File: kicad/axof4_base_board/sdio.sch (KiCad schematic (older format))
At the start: 0 parts

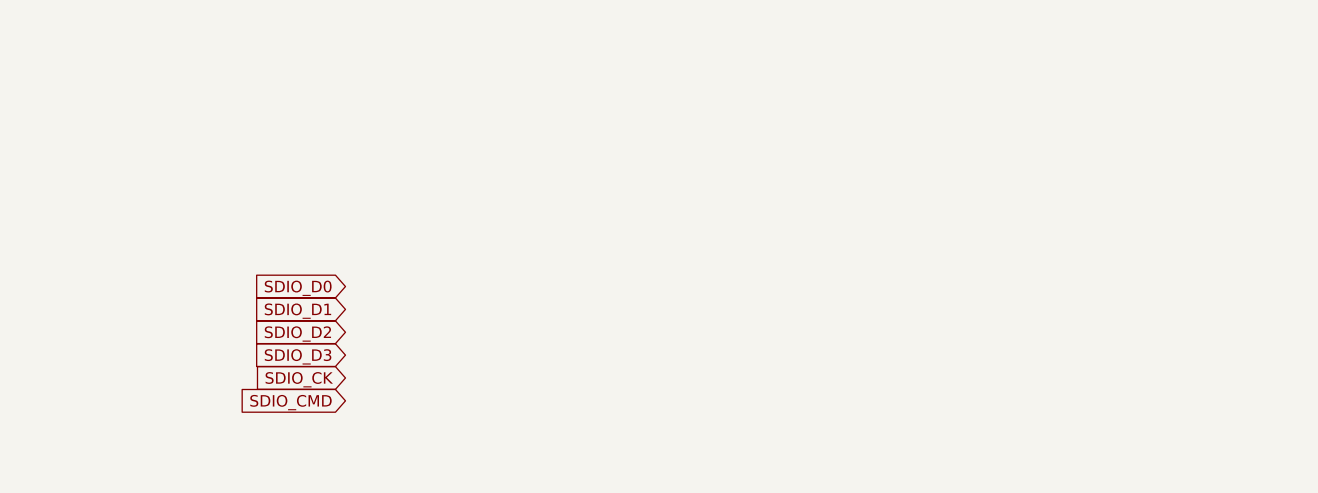
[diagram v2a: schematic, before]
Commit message: cleanup, dedicated PCB WIP
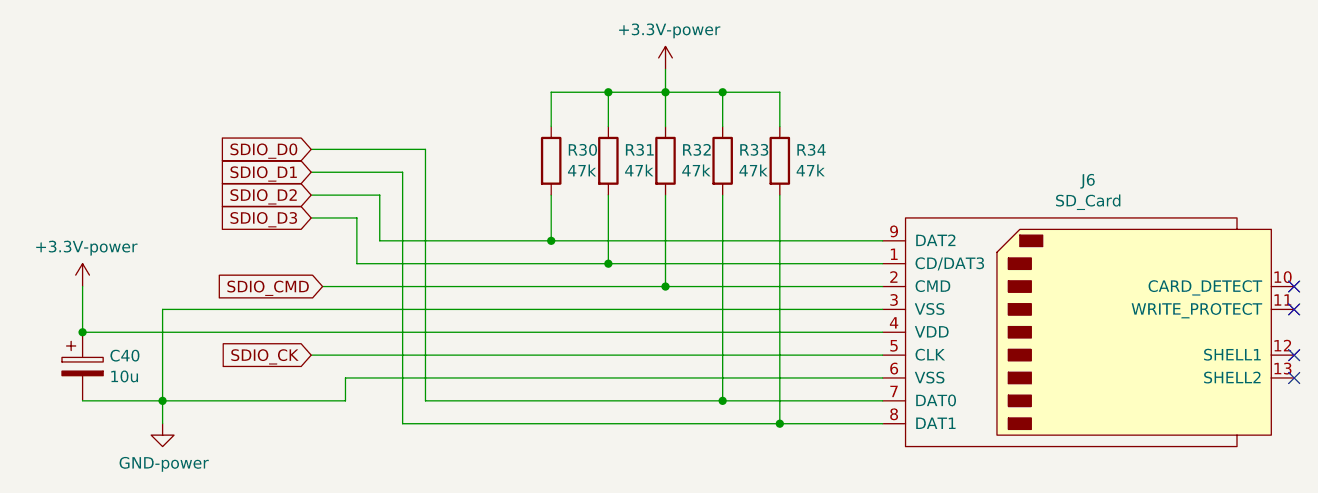
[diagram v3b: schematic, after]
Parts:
- added C40: 10u, Capacitor_SMD:CP_Elec_4x5.4, symbol Device:CP
- added J6: SD_Card, Connector_Card:SD_TE_2041021, symbol Connector:SD_Card
- added R30, R31, R32, R33, R34: 47k, Resistor_SMD:R_1206_3216Metric_Pad1.42x1.75mm_HandSolder, symbol Device:R
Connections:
- net SDIO_CK: now also J6.5 (CLK)
- net SDIO_CMD: now also J6.2 (CMD), R32.2
- net SDIO_D0: now also J6.7 (DAT0), R33.2
- net SDIO_D1: now also J6.8 (DAT1), R34.2
- net SDIO_D2: now also J6.9 (DAT2), R30.2
- net SDIO_D3: now also J6.1 (CD/DAT3), R31.2
- new net +3V3: C40.1, J6.4 (VDD), R30.1, R31.1, R32.1, R33.1, R34.1
- new net GND: C40.2, J6.3 (VSS), J6.6 (VSS)
- no-connect marks 0 -> 4
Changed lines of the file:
@@
 $Descr A4 11693 8268
 encoding utf-8
-Sheet 3 6
+Sheet 3 7
 Title ""
 Date ""
@@
 Comment4 ""
 $EndDescr
-Text GLabel 2500 2700 0    50   Input ~ 0
+Text GLabel 2350 2100 0    50   Input ~ 0
 SDIO_D0
-Text GLabel 2500 2800 0    50   Input ~ 0
+Text GLabel 2350 2200 0    50   Input ~ 0
 SDIO_D1
-Text GLabel 2500 2900 0    50   Input ~ 0
+Text GLabel 2350 2300 0    50   Input ~ 0
 SDIO_D2
-Text GLabel 2500 3000 0    50   Input ~ 0
+Text GLabel 2350 2400 0    50   Input ~ 0
 SDIO_D3
-Text GLabel 2500 3100 0    50   Input ~ 0
+Text GLabel 2400 2700 0    50   Input ~ 0
+SDIO_CMD
+$Comp
+L Connector:SD_Card J6
+U 1 1 5F740056
+P 5750 2900
+F 0 "J6" H 5750 3565 50  0000 C CNN
+F 1 "SD_Card" H 5750 3474 50  0000 C CNN
+F 2 "Connector_Card:SD_TE_2041021" H 5750 2900 50  0001 C CNN
+F 3 "http://portal.fciconnect.com/Comergent//fci/drawing/10067847.pdf" H 5750 2900 50  0001 C CNN
+	1    5750 2900
+	1    0    0    -1
+$EndComp
+Text GLabel 2350 3000 0    50   Input ~ 0
 SDIO_CK
-Text GLabel 2500 3200 0    50   Input ~ 0
-SDIO_CMD
+Wire Wire Line
+	2350 3000 4850 3000
+Wire Wire Line
+	2400 2700 3900 2700
+Wire Wire Line
+	2350 2100 2850 2100
+Wire Wire Line
+	2850 2100 2850 3200
+Wire Wire Line
+	2850 3200 4150 3200
+Wire Wire Line
+	2350 2200 2750 2200
+Wire Wire Line
+	2750 2200 2750 3300
+Wire Wire Line
+	2750 3300 4400 3300
+Wire Wire Line
+	2350 2300 2650 2300
+Wire Wire Line
+	2650 2300 2650 2500
+Wire Wire Line
+	2350 2400 2550 2400
+Wire Wire Line
+	2550 2400 2550 2600
+Wire Wire Line
+	2550 2600 3650 2600
+$Comp
+L axof4_base_board-rescue:+3.3V-power #PWR0103
+U 1 1 5F743FB7
+P 1350 2700
+F 0 "#PWR0103" H 1350 2550 50  0001 C CNN
+F 1 "+3.3V-power" H 1365 2873 50  0000 C CNN
+F 2 "" H 1350 2700 50  0001 C CNN
+F 3 "" H 1350 2700 50  0001 C CNN
+	1    1350 2700
+	1    0    0    -1
+$EndComp
+$Comp
+L axof4_base_board-rescue:GND-power #PWR0104
+U 1 1 5F744B0D
+P 1700 3300
+F 0 "#PWR0104" H 1700 3050 50  0001 C CNN
+F 1 "GND-power" H 1705 3127 50  0000 C CNN
+F 2 "" H 1700 3300 50  0001 C CNN
+F 3 "" H 1700 3300 50  0001 C CNN
+	1    1700 3300
+	1    0    0    -1
+$EndComp
+Wire Wire Line
+	1700 3300 1700 3200
+Wire Wire Line
+	1700 2800 4850 2800
+Wire Wire Line
+	1350 2700 1350 2900
+Wire Wire Line
+	1350 2900 4850 2900
+NoConn ~ 6650 2700
+NoConn ~ 6650 2800
+NoConn ~ 6650 3000
+NoConn ~ 6650 3100
+$Comp
+L Device:CP C40
+U 1 1 5F750B90
+P 1350 3050
+F 0 "C40" H 1468 3096 50  0000 L CNN
+F 1 "10u" H 1468 3005 50  0000 L CNN
+F 2 "Capacitor_SMD:CP_Elec_4x5.4" H 1388 2900 50  0001 C CNN
+F 3 "~" H 1350 3050 50  0001 C CNN
+	1    1350 3050
+	1    0    0    -1
+$EndComp
+Connection ~ 1350 2900
+Wire Wire Line
+	1350 3200 1700 3200
+Connection ~ 1700 3200
+Wire Wire Line
+	1700 2800 1700 3200
+Wire Wire Line
+	1700 3200 2500 3200
+Wire Wire Line
+	2500 3200 2500 3100
+Wire Wire Line
+	2500 3100 4850 3100
+$Comp
+L Device:R R30
+U 1 1 5F753A6C
+P 3400 2150
+F 0 "R30" H 3470 2196 50  0000 L CNN
+F 1 "47k" H 3470 2105 50  0000 L CNN
+F 2 "Resistor_SMD:R_1206_3216Metric_Pad1.42x1.75mm_HandSolder" V 3330 2150 50  0001 C CNN
+F 3 "~" H 3400 2150 50  0001 C CNN
+	1    3400 2150
+	1    0    0    -1
+$EndComp
+$Comp
+L Device:R R31
+U 1 1 5F757136
+P 3650 2150
+F 0 "R31" H 3720 2196 50  0000 L CNN
+F 1 "47k" H 3720 2105 50  0000 L CNN
+F 2 "Resistor_SMD:R_1206_3216Metric_Pad1.42x1.75mm_HandSolder" V 3580 2150 50  0001 C CNN
+F 3 "~" H 3650 2150 50  0001 C CNN
+	1    3650 2150
+	1    0    0    -1
+$EndComp
+$Comp
+L Device:R R32
+U 1 1 5F75727F
+P 3900 2150
+F 0 "R32" H 3970 2196 50  0000 L CNN
+F 1 "47k" H 3970 2105 50  0000 L CNN
+F 2 "Resistor_SMD:R_1206_3216Metric_Pad1.42x1.75mm_HandSolder" V 3830 2150 50  0001 C CNN
+F 3 "~" H 3900 2150 50  0001 C CNN
+	1    3900 2150
+	1    0    0    -1
+$EndComp
+$Comp
+L Device:R R33
+U 1 1 5F757554
+P 4150 2150
+F 0 "R33" H 4220 2196 50  0000 L CNN
+F 1 "47k" H 4220 2105 50  0000 L CNN
+F 2 "Resistor_SMD:R_1206_3216Metric_Pad1.42x1.75mm_HandSolder" V 4080 2150 50  0001 C CNN
+F 3 "~" H 4150 2150 50  0001 C CNN
+	1    4150 2150
+	1    0    0    -1
+$EndComp
+$Comp
+L Device:R R34
+U 1 1 5F7577B3
+P 4400 2150
+F 0 "R34" H 4470 2196 50  0000 L CNN
+F 1 "47k" H 4470 2105 50  0000 L CNN
+F 2 "Resistor_SMD:R_1206_3216Metric_Pad1.42x1.75mm_HandSolder" V 4330 2150 50  0001 C CNN
+F 3 "~" H 4400 2150 50  0001 C CNN
+	1    4400 2150
+	1    0    0    -1
+$EndComp
+Wire Wire Line
+	3650 2300 3650 2600
+Connection ~ 3650 2600
+Wire Wire Line
+	3650 2600 4850 2600
+Wire Wire Line
+	2650 2500 3400 2500
+Wire Wire Line
+	3400 2300 3400 2500
+Connection ~ 3400 2500
+Wire Wire Line
+	3400 2500 4850 2500
+Wire Wire Line
+	3900 2300 3900 2700
+Connection ~ 3900 2700
+Wire Wire Line
+	3900 2700 4850 2700
+Wire Wire Line
+	4150 2300 4150 3200
+Connection ~ 4150 3200
+Wire Wire Line
+	4150 3200 4850 3200
+Wire Wire Line
+	4400 2300 4400 3300
+Connection ~ 4400 3300
+Wire Wire Line
+	4400 3300 4850 3300
+$Comp
+L axof4_base_board-rescue:+3.3V-power #PWR0105
+U 1 1 5F75AFEC
+P 3900 1750
+F 0 "#PWR0105" H 3900 1600 50  0001 C CNN
+F 1 "+3.3V-power" H 3915 1923 50  0000 C CNN
+F 2 "" H 3900 1750 50  0001 C CNN
+F 3 "" H 3900 1750 50  0001 C CNN
+	1    3900 1750
+	1    0    0    -1
+$EndComp
+Wire Wire Line
+	3400 2000 3400 1850
+Wire Wire Line
+	3400 1850 3650 1850
+Wire Wire Line
+	3900 1850 3900 1750
+Wire Wire Line
+	3900 1850 4150 1850
+Wire Wire Line
+	4400 1850 4400 2000
+Connection ~ 3900 1850
+Wire Wire Line
+	3650 2000 3650 1850
+Connection ~ 3650 1850
+Wire Wire Line
+	3650 1850 3900 1850
+Wire Wire Line
+	3900 2000 3900 1850
+Wire Wire Line
+	4150 2000 4150 1850
+Connection ~ 4150 1850
+Wire Wire Line
+	4150 1850 4400 1850
 $EndSCHEMATC

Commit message: rollback kicad project to use STM32F4DISCOVERY
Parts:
- C40: footprint Capacitor_SMD:CP_Elec_4x5.4 -> Capacitor_SMD:CP_Elec_6.3x5.3
- R30, R31, R32, R33, R34: footprint Resistor_SMD:R_1206_3216Metric_Pad1.42x1.75mm_HandSolder -> Resistor_SMD:R_0603_1608Metric
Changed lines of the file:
@@
 F 0 "C40" H 1468 3096 50  0000 L CNN
 F 1 "10u" H 1468 3005 50  0000 L CNN
-F 2 "Capacitor_SMD:CP_Elec_4x5.4" H 1388 2900 50  0001 C CNN
+F 2 "Capacitor_SMD:CP_Elec_6.3x5.3" H 1388 2900 50  0001 C CNN
 F 3 "~" H 1350 3050 50  0001 C CNN
 	1    1350 3050
@@
 F 0 "R30" H 3470 2196 50  0000 L CNN
 F 1 "47k" H 3470 2105 50  0000 L CNN
-F 2 "Resistor_SMD:R_1206_3216Metric_Pad1.42x1.75mm_HandSolder" V 3330 2150 50  0001 C CNN
+F 2 "Resistor_SMD:R_0603_1608Metric" V 3330 2150 50  0001 C CNN
 F 3 "~" H 3400 2150 50  0001 C CNN
 	1    3400 2150
@@
 F 0 "R31" H 3720 2196 50  0000 L CNN
 F 1 "47k" H 3720 2105 50  0000 L CNN
-F 2 "Resistor_SMD:R_1206_3216Metric_Pad1.42x1.75mm_HandSolder" V 3580 2150 50  0001 C CNN
+F 2 "Resistor_SMD:R_0603_1608Metric" V 3580 2150 50  0001 C CNN
 F 3 "~" H 3650 2150 50  0001 C CNN
 	1    3650 2150
@@
 F 0 "R32" H 3970 2196 50  0000 L CNN
 F 1 "47k" H 3970 2105 50  0000 L CNN
-F 2 "Resistor_SMD:R_1206_3216Metric_Pad1.42x1.75mm_HandSolder" V 3830 2150 50  0001 C CNN
+F 2 "Resistor_SMD:R_0603_1608Metric" V 3830 2150 50  0001 C CNN
 F 3 "~" H 3900 2150 50  0001 C CNN
 	1    3900 2150
@@
 F 0 "R33" H 4220 2196 50  0000 L CNN
 F 1 "47k" H 4220 2105 50  0000 L CNN
-F 2 "Resistor_SMD:R_1206_3216Metric_Pad1.42x1.75mm_HandSolder" V 4080 2150 50  0001 C CNN
+F 2 "Resistor_SMD:R_0603_1608Metric" V 4080 2150 50  0001 C CNN
 F 3 "~" H 4150 2150 50  0001 C CNN
 	1    4150 2150
@@
 F 0 "R34" H 4470 2196 50  0000 L CNN
 F 1 "47k" H 4470 2105 50  0000 L CNN
-F 2 "Resistor_SMD:R_1206_3216Metric_Pad1.42x1.75mm_HandSolder" V 4330 2150 50  0001 C CNN
+F 2 "Resistor_SMD:R_0603_1608Metric" V 4330 2150 50  0001 C CNN
 F 3 "~" H 4400 2150 50  0001 C CNN
 	1    4400 2150
